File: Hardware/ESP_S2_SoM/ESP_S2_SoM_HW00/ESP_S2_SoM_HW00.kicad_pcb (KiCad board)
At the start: 6 copper layers, 29.5 x 24.7 mm, 55 parts, among them J1 DF40C-60DP-0.4V(51), J2 Bare PCB USB C, SW401 SW_Push, SW402 SW_Push, U201 BQ24075RGTR, U301 MIC5528-3.3YMT-T5, U401 ESP32-S2FH4, Y601 Crystal_GND24_Small

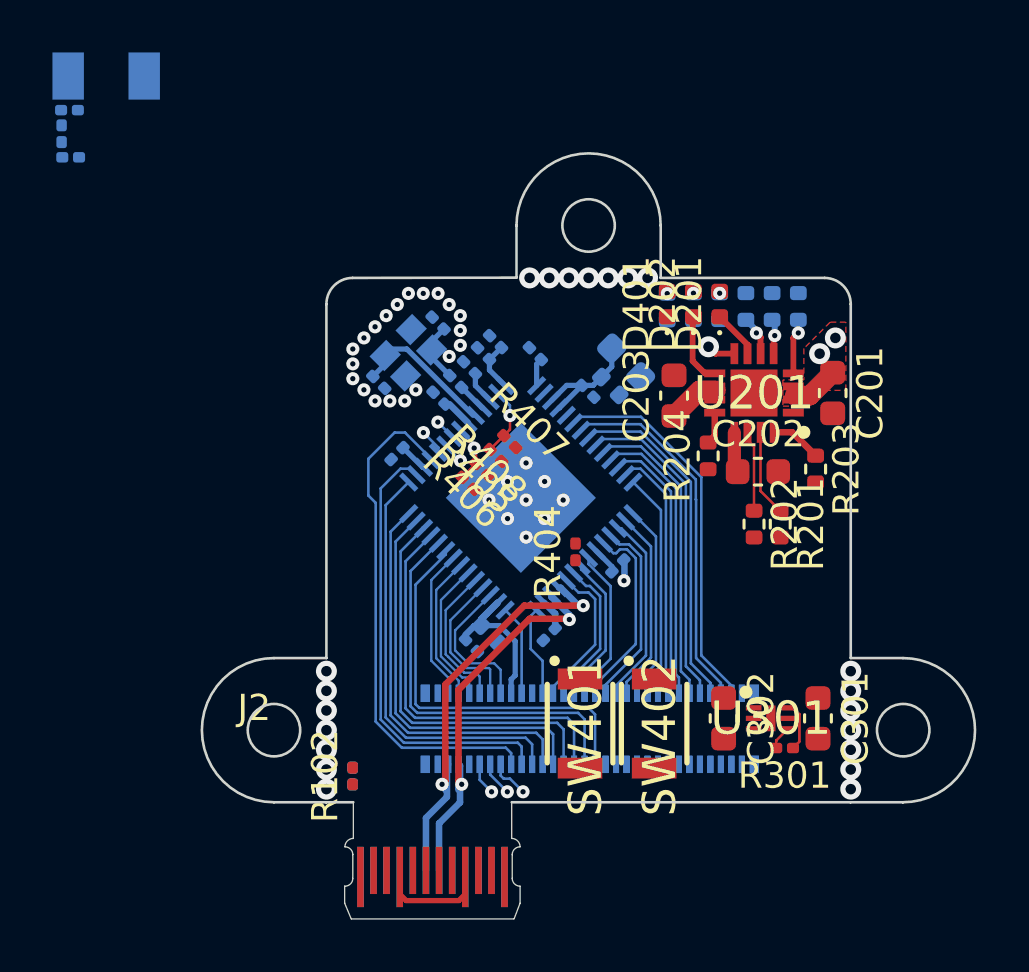
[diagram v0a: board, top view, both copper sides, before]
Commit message: ESP32 data is done
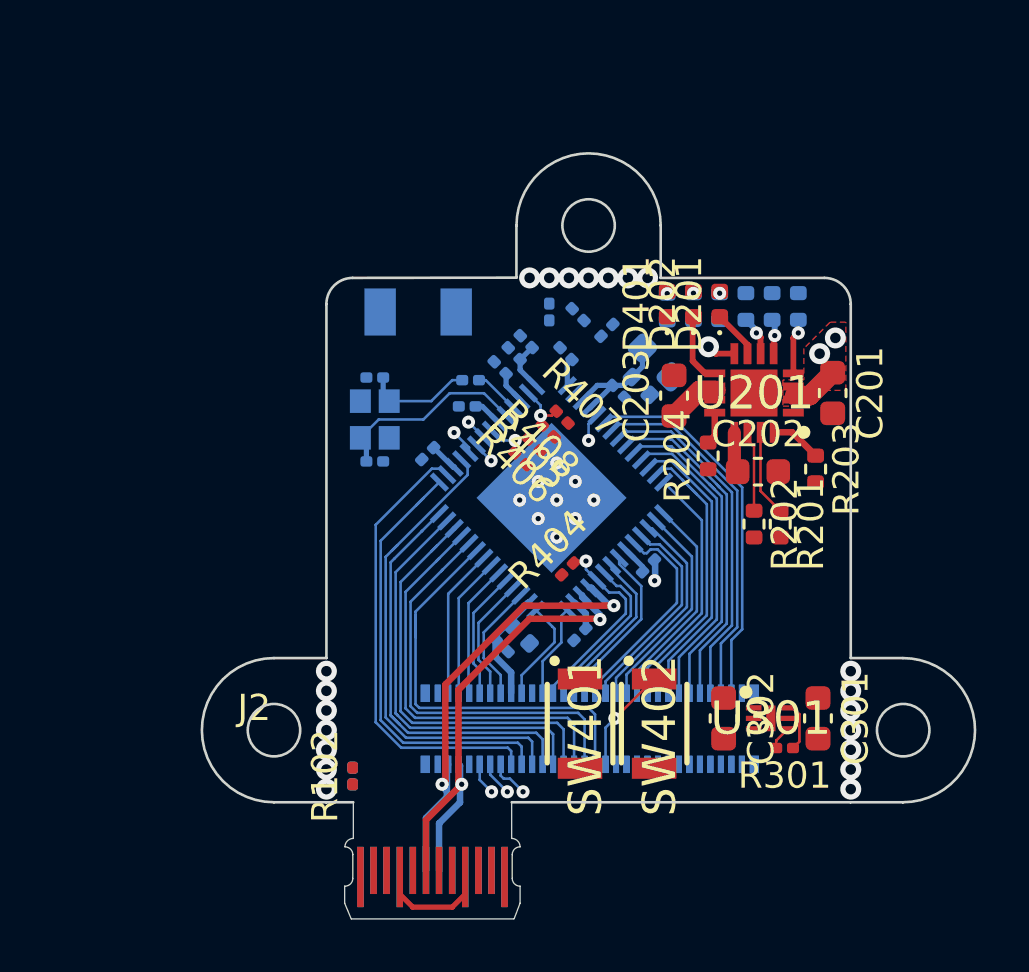
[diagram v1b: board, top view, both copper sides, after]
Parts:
- moved C407 21.5 mm to (136.7, 91.0), turned to 45 degrees
- moved L401 20.9 mm to (135.6, 90.4), turned to -45 degrees
- moved C406 19.9 mm to (134.5, 90.3), turned to -90 degrees
- moved ANT401 14.9 mm to (129.5, 90.3), turned to 180 degrees
- moved C401 3.19 mm to (127.8, 92.8), turned to 180 degrees
- moved C402 3.02 mm to (127.8, 96.0), turned to 0 degrees
- moved Y601 2.85 mm to (127.8, 94.4), turned to 90 degrees
- moved R406 2.21 mm to (133.9, 95.4)
- moved R405 2.21 mm to (134.5, 94.8)
- moved R407 2.21 mm to (135.0, 94.3)
- moved R408 2.21 mm to (133.4, 95.9)
- moved C410 1.17 mm to (138.0, 93.1)
- moved C403 1.17 mm to (129.9, 95.7)
- moved C404 1.17 mm to (132.6, 92.4)
- moved C408 1.17 mm to (135.1, 91.9)
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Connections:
- J1 pad 42: IO39 -> IO41 (x2)
- J1 pad 44: IO40 -> IO39 (x2)
- J1 pad 46: IO41 -> IO40 (x2)
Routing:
- net IO0: track 0.00 -> 16.7 mm, vias 0 -> 2
- net /100_Connectors/D+: track 14.9 -> 19.9 mm
- net Net-(C401-Pad1): track 1.98 -> 4.11 mm
- net Net-(U401-XTAL_N): track 5.15 -> 7.28 mm
- net IO18: track 5.65 -> 7.55 mm, vias 0 -> 1
- net IO8: track 9.76 -> 11.3 mm
- net SPI6: track 8.13 -> 6.59 mm
- net IO33: track 15.2 -> 16.6 mm
- net /100_Connectors/D-: track 16.2 -> 17.4 mm
- net IO41: track 19.5 -> 18.3 mm
- net SPI5: track 5.61 -> 4.60 mm
- net IO38: track 15.1 -> 16.1 mm
- net SPI4: track 5.68 -> 4.77 mm
- net IO5: track 11.7 -> 12.5 mm
- net IO14: track 7.39 -> 8.20 mm
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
